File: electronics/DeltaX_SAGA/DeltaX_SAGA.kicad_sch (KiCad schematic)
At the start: 73 parts, among them J1 USB_B_Micro, J10 Motor3_Encoder, J11 M12, J12 M21, J13 M22, J14 M31, J15 M33, J16 Thrower+, J17 Thrower-, J2 Programmer, J3 SERVO, J4 M11, J5 Battery+, J6 Thrower Signal, J7 Battery-, J8 Motor1_Encoder, J9 Motor2_Encoder, Q1 BUK6Y10, U1 CM1223, U10 DRV8243, U11 DRV8243, U2 NCP164C, U3 STM32G441KB, U5 TPS62933, U6 MAX14930, U7 MAX14930, U8 MAX12930, U9 DRV8243

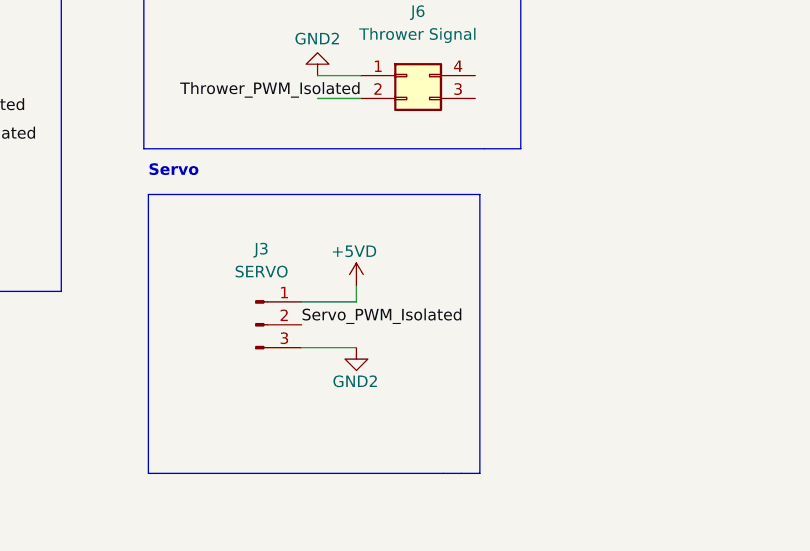
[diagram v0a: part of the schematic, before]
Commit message: Schematic updated
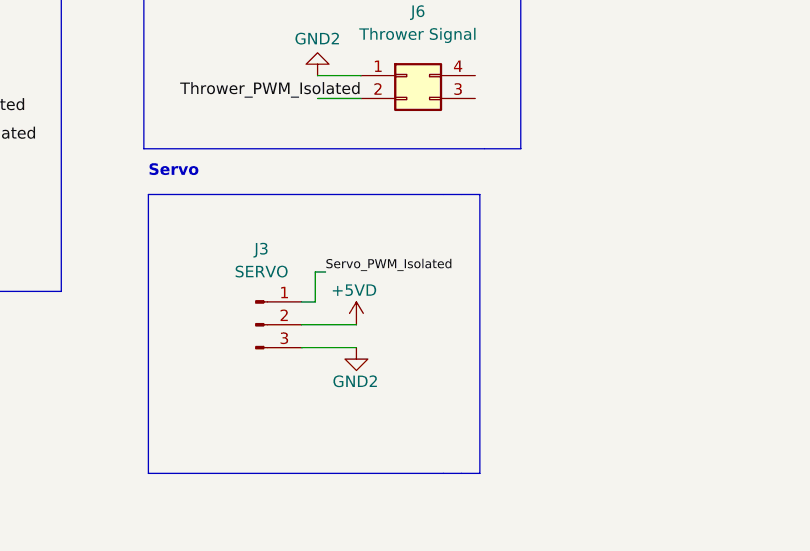
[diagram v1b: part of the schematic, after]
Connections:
- net +5VD: now also J3.2 (Pin_2); no longer J3.1 (Pin_1)
- net Servo_PWM_Isolated: now also J3.1 (Pin_1); no longer J3.2 (Pin_2)
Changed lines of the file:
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@@
     (stroke (width 0) (type default) (color 0 0 0 0))
   )
-  (wire (pts (xy 343.408 228.6) (xy 343.408 226.822))
+  (wire (pts (xy 338.836 228.6) (xy 338.836 225.2726))
     (stroke (width 0) (type default) (color 0 0 0 0))
   )
@@
     (stroke (width 0) (type default) (color 0 0 0 0))
   )
-  (wire (pts (xy 337.312 228.6) (xy 343.408 228.6))
+  (wire (pts (xy 337.312 231.14) (xy 343.408 231.14))
     (stroke (width 0) (type default) (color 0 0 0 0))
   )
@@
     (stroke (width 0) (type default) (color 0 0 0 0))
   )
+  (wire (pts (xy 338.836 225.2726) (xy 339.979 225.2726))
+    (stroke (width 0) (type default) (color 0 0 0 0))
+  )
   (wire (pts (xy 345.821 82.3976) (xy 345.821 84.963))
     (stroke (width 0) (type default) (color 0 0 0 0))
@@
   )
   (polyline (pts (xy 390.017 174.625) (xy 390.017 147.574))
+    (stroke (width 0) (type default) (color 0 0 0 0))
+  )
+  (wire (pts (xy 337.312 228.6) (xy 338.836 228.6))
     (stroke (width 0) (type default) (color 0 0 0 0))
   )
@@
     (effects (font (size 1.27 1.27)) (justify left bottom))
   )
-  (label "Servo_PWM_Isolated" (at 337.312 231.14 0)
-    (effects (font (size 1.27 1.27)) (justify left bottom))
+  (label "Servo_PWM_Isolated" (at 339.979 225.2726 0)
+    (effects (font (size 1 1)) (justify left bottom))
   )
   (label "Motor3_OUT1" (at 289.3568 41.7322 180)
@@
     (pin "2")
   )
-  (symbol (lib_id "power:+5VD") (at 343.408 226.822 0) (unit 1)
-    (in_bom yes) (on_board yes)
-    (property "Reference" "#PWR014" (id 0) (at 343.408 230.632 0)
-      (effects (font (size 1.27 1.27)) hide)
-    )
-    (property "Value" "+5VD" (id 1) (at 343.154 223.012 0))
-    (property "Footprint" "" (id 2) (at 343.408 226.822 0)
-      (effects (font (size 1.27 1.27)) hide)
-    )
-    (property "Datasheet" "" (id 3) (at 343.408 226.822 0)
-      (effects (font (size 1.27 1.27)) hide)
-    )
+  (symbol (lib_id "power:+5VD") (at 343.408 231.14 0) (unit 1)
+    (in_bom yes) (on_board yes)
+    (property "Reference" "#PWR014" (id 0) (at 343.408 234.95 0)
+      (effects (font (size 1.27 1.27)) hide)
+    )
+    (property "Value" "+5VD" (id 1) (at 343.154 227.33 0))
+    (property "Footprint" "" (id 2) (at 343.408 231.14 0)
+      (effects (font (size 1.27 1.27)) hide)
+    )
+    (property "Datasheet" "" (id 3) (at 343.408 231.14 0)
+      (effects (font (size 1.27 1.27)) hide)
+    )
